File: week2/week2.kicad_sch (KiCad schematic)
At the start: 18 parts, among them J1 PJ-102AH, J2 Conn_01x06, SW1 Omron_B3F_SPST, U1 ATmega328-PU, U2 L7805, Y1 Crystal_16MHz

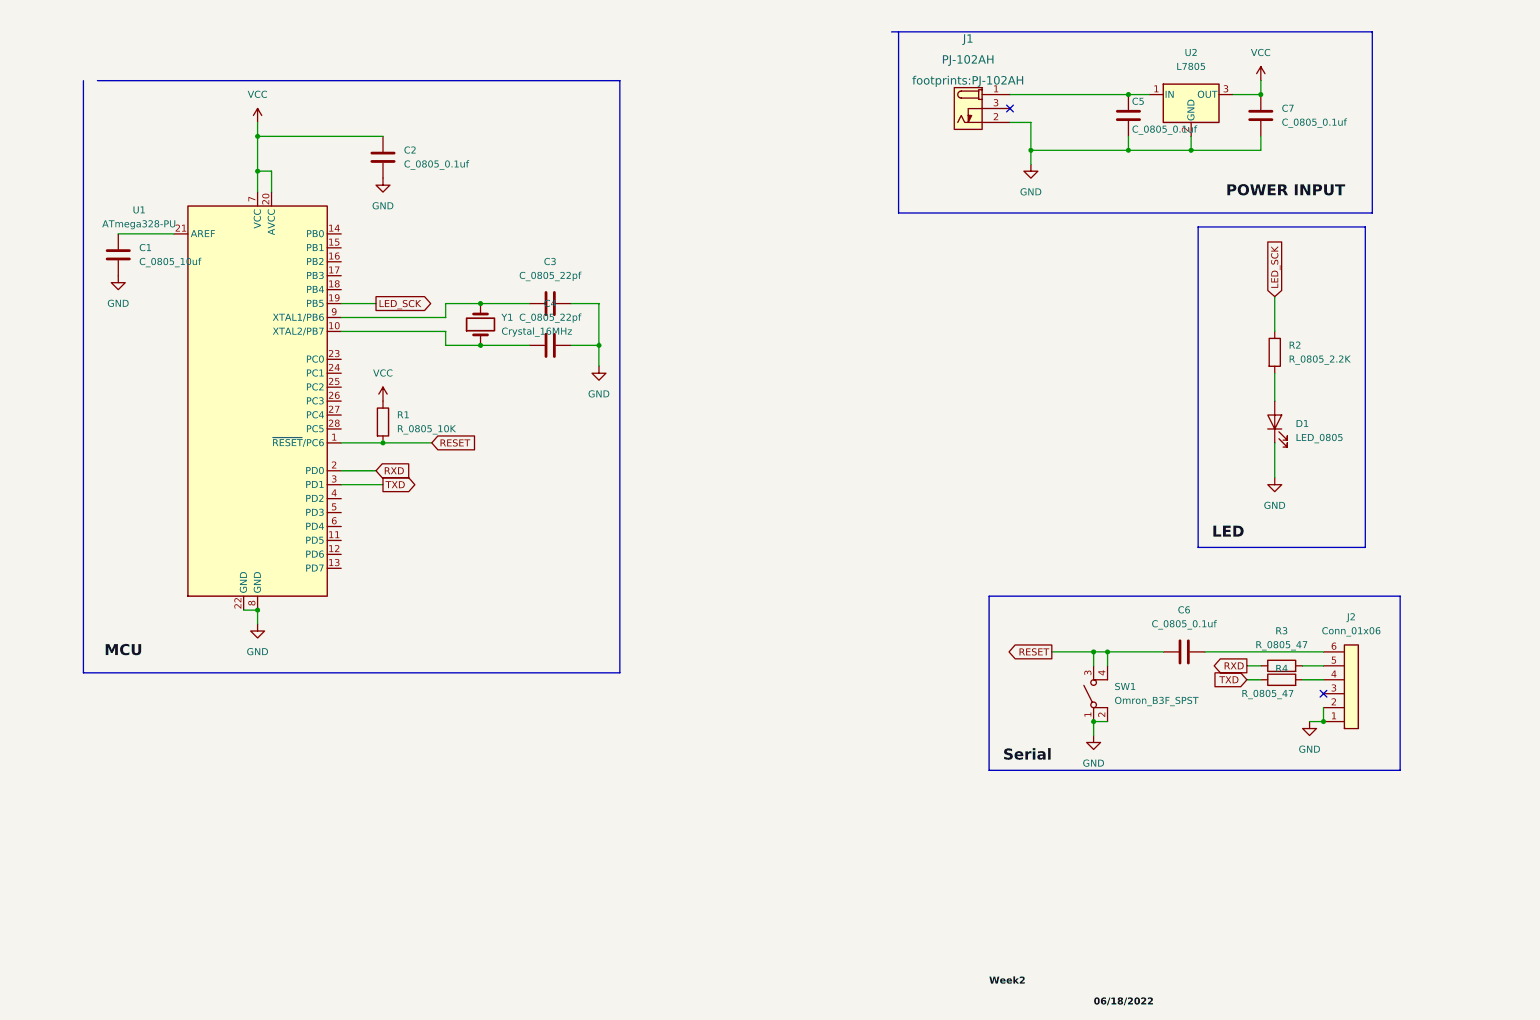
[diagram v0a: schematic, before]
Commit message: schematic review
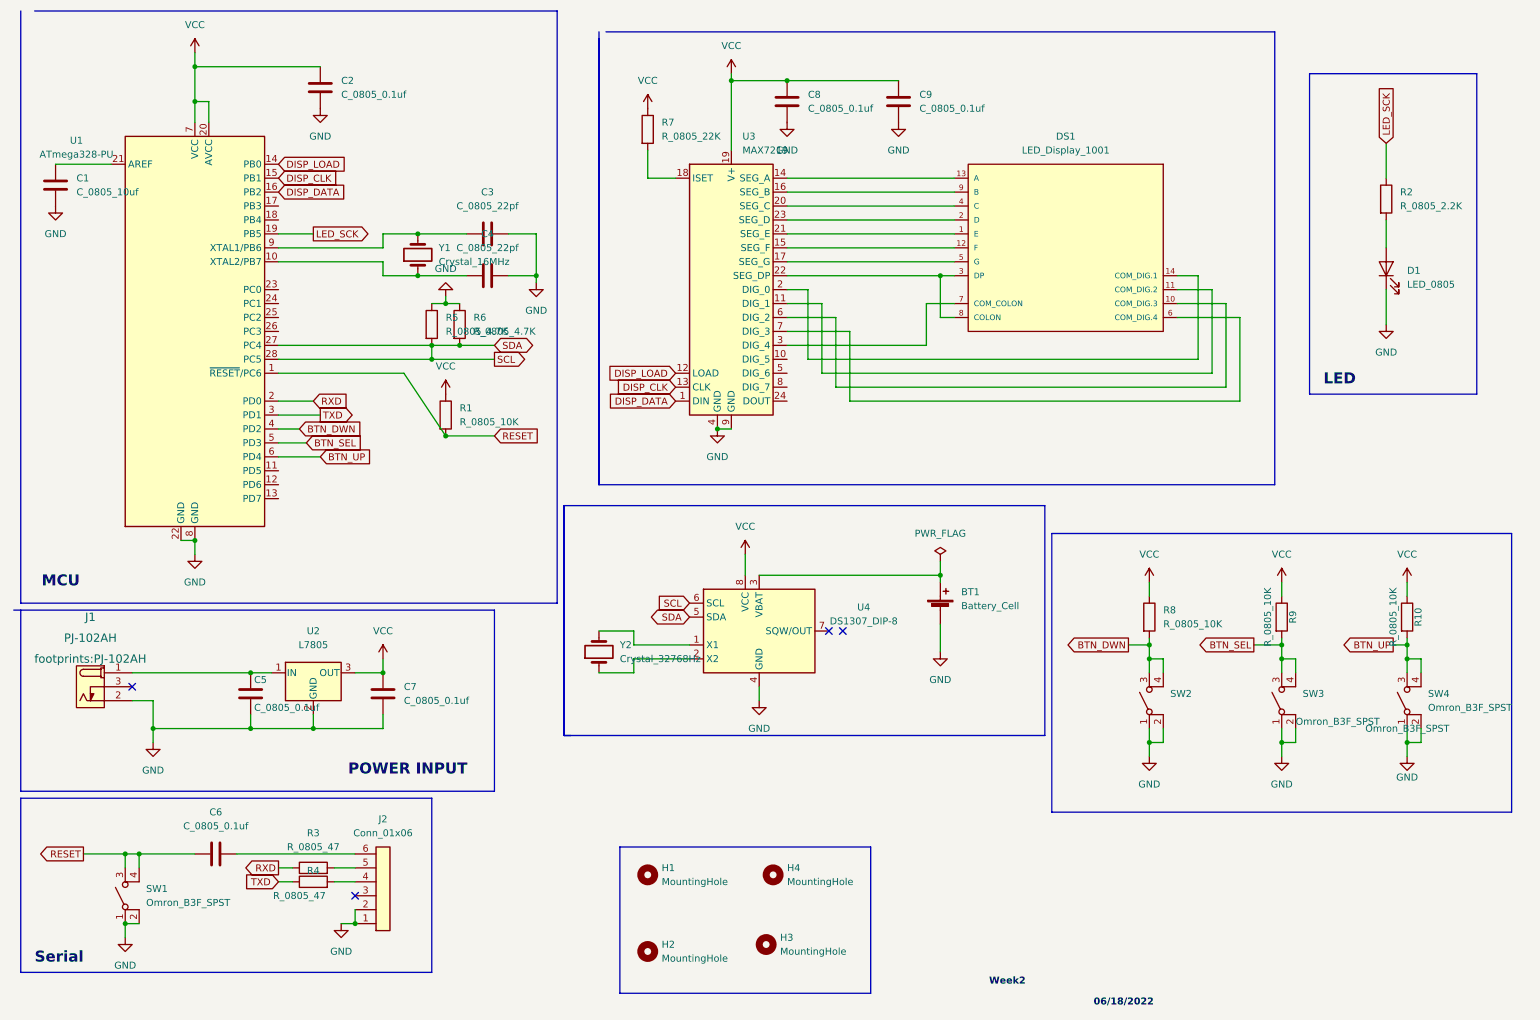
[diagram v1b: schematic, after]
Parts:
- added BT1: Battery_Cell, footprints:BatteryHolder_Keystone_106_1x20mm, symbol HPS:Battery_Cell
- added C8, C9: C_0805_0.1uf, footprints:C_0805_2012Metric, symbol HPS:C_0805_0.1uf
- added DS1: LED_Display_1001, footprints:Adafruit-1001-0-0-MFG, symbol HPS:LED_Display_1001
- added H1, H2, H3, H4: MountingHole, footprints:MountingHole_3.2mm_M3, symbol HPS:MountingHole
- added R10, R8, R9: R_0805_10K, footprints:R_0805_2012Metric, symbol HPS:R_0805_10K
- added R5, R6: R_0805_4.7K, footprints:R_0805_2012Metric, symbol HPS:R_0805_4.7K
- added R7: R_0805_22K, footprints:R_0805_2012Metric, symbol HPS:R_0805_22K
- added SW2, SW3, SW4: Omron_B3F_SPST, footprints:SW_SPST_Omron_B3FS-100xP, symbol HPS:Omron_B3F_SPST
- added U3: MAX7219, footprints:DIP-24_W7.62mm, symbol HPS:MAX7219
- added U4: DS1307_DIP-8, footprints:DIP-8_W7.62mm, symbol HPS:DS1307_DIP-8
- added Y2: Crystal_32768Hz, footprints:Crystal_SMD_2Pin_3.2x1.5mm, symbol HPS:Crystal_32768Hz
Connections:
- net GND: now also BT1.2 (-), C8.1, C9.2, R5.1, R6.1, SW2.1 (A), SW2.2 (A), SW3.1 (A), SW3.2 (A), SW4.1 (A), SW4.2 (A), U3.4 (GND), U3.9 (GND), U4.4 (GND)
- net VCC: now also C8.2, C9.1, R10.1, R7.1, R8.1, R9.1, U3.19 (V+), U4.8 (VCC)
- net DISP_LOAD: now reaches U1.14 (PB0)
- net DISP_LOAD: now also U3.12 (LOAD)
- net DISP_CLK: now reaches U1.15 (PB1)
- net DISP_CLK: now also U3.13 (CLK)
- net DISP_DATA: now reaches U1.16 (PB2)
- net DISP_DATA: now also U3.1 (DIN)
- net SCL: now reaches U1.27 (PC4)
- net SCL: now also U1.28 (PC5), R5.2, R6.2, U4.5 (SDA), U4.6 (SCL)
- net BTN_DWN: now reaches U1.4 (PD2)
- net BTN_DWN: now also R8.2, SW2.3 (B), SW2.4 (B)
- net BTN_SEL: now reaches U1.5 (PD3)
- net BTN_SEL: now also R9.2, SW3.3 (B), SW3.4 (B)
- net BTN_UP: now reaches U1.6 (PD4)
- net BTN_UP: now also R10.2, SW4.3 (B), SW4.4 (B)
- new net: DS1.1 (E), U3.21 (SEG_E)
- new net: DS1.10 (COM_DIG.3), U3.6 (DIG_2)
- new net: DS1.11 (COM_DIG.2), U3.11 (DIG_1)
- new net: DS1.12 (F), U3.15 (SEG_F)
- new net: DS1.13 (A), U3.14 (SEG_A)
- new net: DS1.14 (COM_DIG.1), U3.2 (DIG_0)
- new net: DS1.2 (D), U3.23 (SEG_D)
- new net: DS1.3 (DP), DS1.8 (COLON), U3.22 (SEG_DP)
- new net: DS1.4 (C), U3.20 (SEG_C)
- new net: DS1.5 (G), U3.17 (SEG_G)
- new net: DS1.6 (COM_DIG.4), U3.7 (DIG_3)
- new net: DS1.7 (COM_COLON), U3.3 (DIG_4)
- new net: DS1.9 (B), U3.16 (SEG_B)
- new net: U4.1 (X1), Y2.2
- new net: U4.2 (X2), Y2.1
- new net: BT1.1 (+), U4.3 (VBAT)
- new net: R7.2, U3.18 (ISET)
- no-connect marks 2 -> 4
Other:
- moved on the sheet: C1, C2, C3, C4, C5, C6, C7, D1, J1, J2, R1, R2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
